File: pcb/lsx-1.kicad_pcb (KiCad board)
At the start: 2 copper layers, 25.4 x 27.9 mm, 7 parts, among them J1 RJ45, J2 USART-USB, J3 ISP

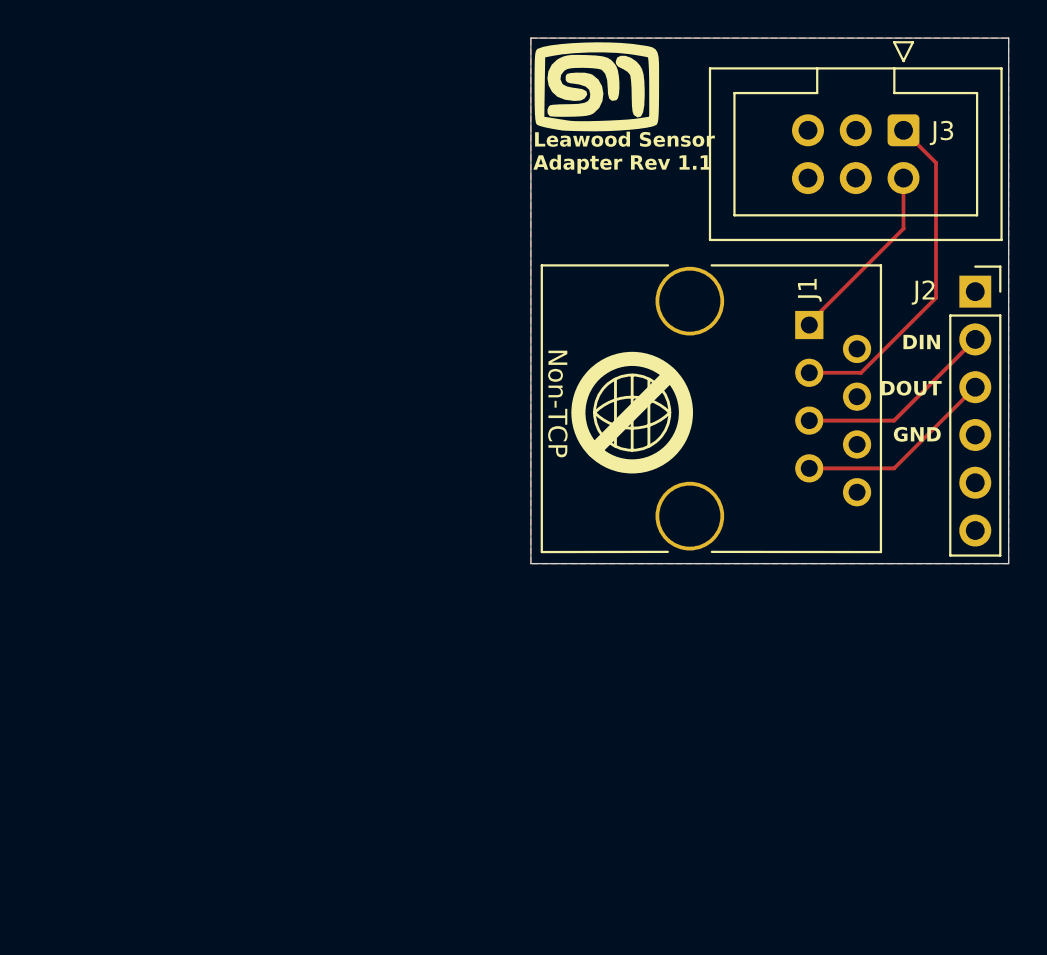
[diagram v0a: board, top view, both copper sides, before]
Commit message: Update
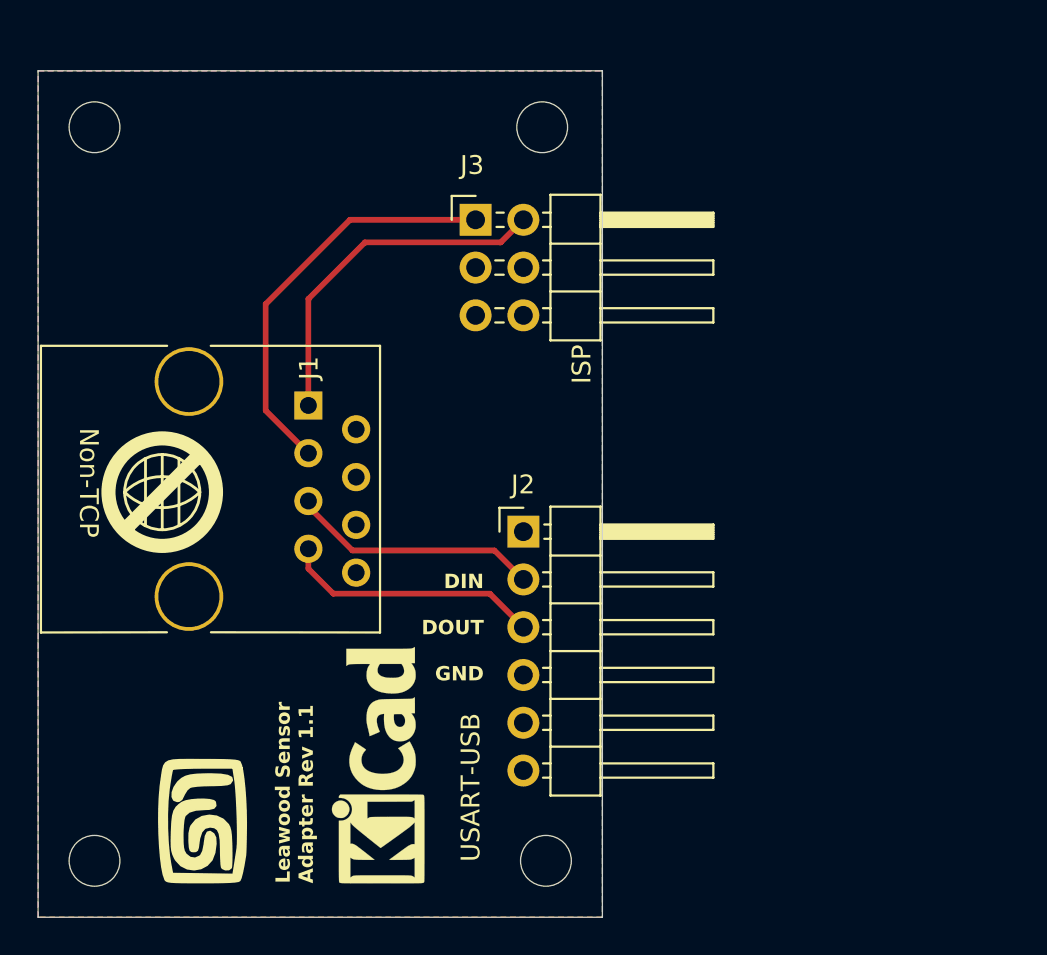
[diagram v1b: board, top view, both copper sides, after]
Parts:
- added H1: MountingHole, MountingHole:MountingHole_2.7mm_M2.5, F.Cu at (53.0, 53.0)
- added H2: MountingHole, MountingHole:MountingHole_2.7mm_M2.5, F.Cu at (53.0, 92.0)
- added H3: MountingHole, MountingHole:MountingHole_2.7mm_M2.5, F.Cu at (77.0, 92.0)
- added H4: MountingHole, MountingHole:MountingHole_2.7mm_M2.5, F.Cu at (76.8, 53.0)
- J2: footprint Connector_PinSocket_2.54mm:PinSocket_1x06_P2.54mm_Vertical -> Connector_PinHeader_2.54mm:PinHeader_1x06_P2.54mm_Horizontal
- J3: footprint Connector_IDC:IDC-Header_2x03_P2.54mm_Vertical -> Connector_PinHeader_2.54mm:PinHeader_2x03_P2.54mm_Horizontal
- Lg2: moved to F.Cu
- moved Lg1 44.4 mm to (58.7, 89.9), turned to 90 degrees
- moved Lg2 32.6 mm to (68.6, 86.9), turned to 90 degrees
- moved J2 27.2 mm to (75.8, 74.5)
- moved J1 27.0 mm to (66.9, 76.7)
- moved Lg3 25.3 mm to (56.6, 72.4)
- moved Lg4 25.3 mm to (56.6, 72.4)
- moved J3 23.2 mm to (73.3, 57.9), turned to 0 degrees
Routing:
- net +3.3V: track 9.89 -> 18.8 mm
- net /UPDI: track 18.0 -> 21.9 mm
- net /DOUT: track 10.6 -> 13.8 mm
- net /DIN: track 10.6 -> 13.3 mm
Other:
- board size 25.4 x 27.9 mm -> 30 x 45 mm
- board text removed: "UPDI 3V3"
